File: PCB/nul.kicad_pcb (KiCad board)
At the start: 2 copper layers, 10 x 40 mm, 33 parts, among them J2 LED Socket, U1 ESP32-C3FH4, U2 AMS1117-3.3, U3 SN74AHCT1G125DBVR, U4 XRCGB40M000F1S1DR0, U5 SRV05-4

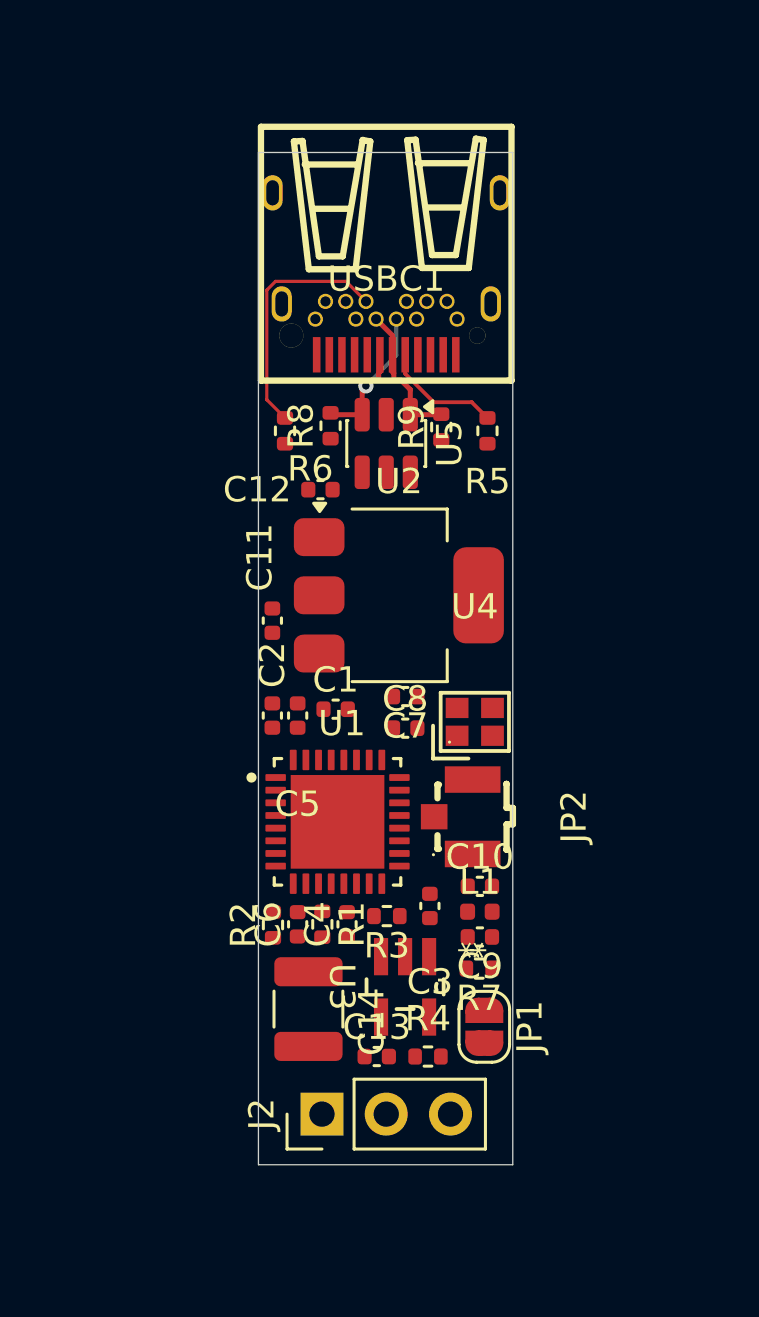
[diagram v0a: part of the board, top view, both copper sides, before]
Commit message: pcb v1
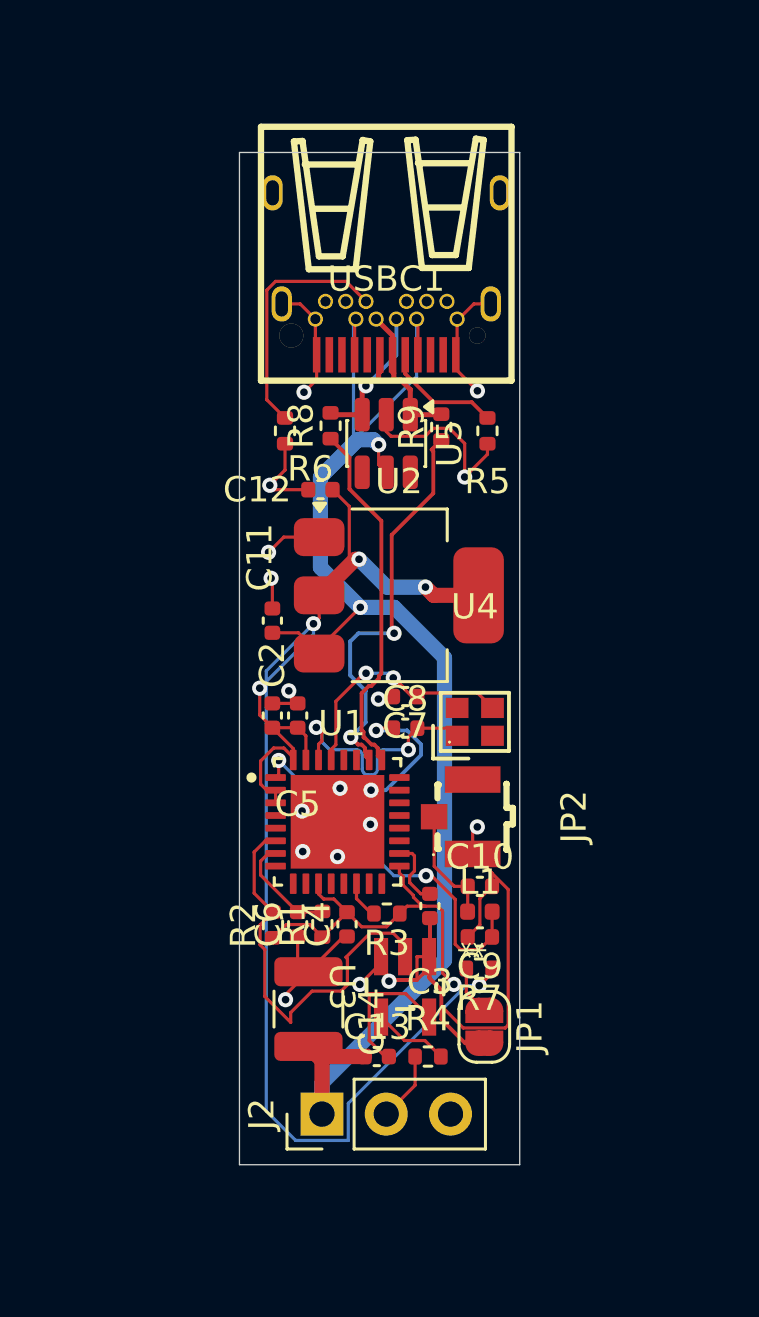
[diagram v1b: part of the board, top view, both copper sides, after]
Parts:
- removed C1: 0.1uF ceramic, Capacitor_SMD:C_0402_1005Metric
- moved R3 0.10 mm to (120.0, 70.1)
- turned R1 to 90 degrees
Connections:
- net Net-(U1-GPIO18/USB_D-) renamed /USB_DATA+
- net Net-(U1-GPIO19/USB_D+) renamed /USB_DATA-
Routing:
- net +3.3V: track 0.00 -> 75.9 mm, vias 0 -> 6
- net GND: track 0.00 -> 68.9 mm, vias 0 -> 19
- net +5V: track 0.00 -> 57.3 mm, vias 0 -> 2
- net /USB_DATA-: track 0.00 -> 16.0 mm, vias 0 -> 2
- net LED: track 0.00 -> 15.9 mm
- net Net-(U1-LNA_IN): track 0.00 -> 14.5 mm, vias 0 -> 2
- net /USB_DATA+: track 0.00 -> 14.3 mm
- net Net-(U1-XTAL_P): track 0.00 -> 9.46 mm, vias 0 -> 2
- net Net-(U1-XTAL_N): track 0.00 -> 9.34 mm, vias 0 -> 2
- net Net-(U3-VCC): track 0.00 -> 5.50 mm
- net Net-(JP2-SIG): track 0.00 -> 4.60 mm
- net Net-(U1-CHIP_EN): track 0.00 -> 4.00 mm
- net Net-(U3-Y): track 0.00 -> 3.01 mm
- net Net-(U1-VDD_SPI): track 0.00 -> 2.75 mm
- net Net-(J2-Pin_2): track 0.00 -> 2.75 mm
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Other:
- board size 10 x 40 mm -> 11.1 x 40 mm
